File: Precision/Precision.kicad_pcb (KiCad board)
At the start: 2 copper layers, 76.2 x 76.2 mm, 159 parts, among them J1 M04PTH, J2 M04PTH, J3 M06SIP, J4 M04PTH, J405 Conn_01x08, J406 Conn_01x08, J5 M06SIP, J6 M02PTH, U401 ATMEGA328P-AU, U501 FT232RL, U602 ZF7, Y401 16MHz

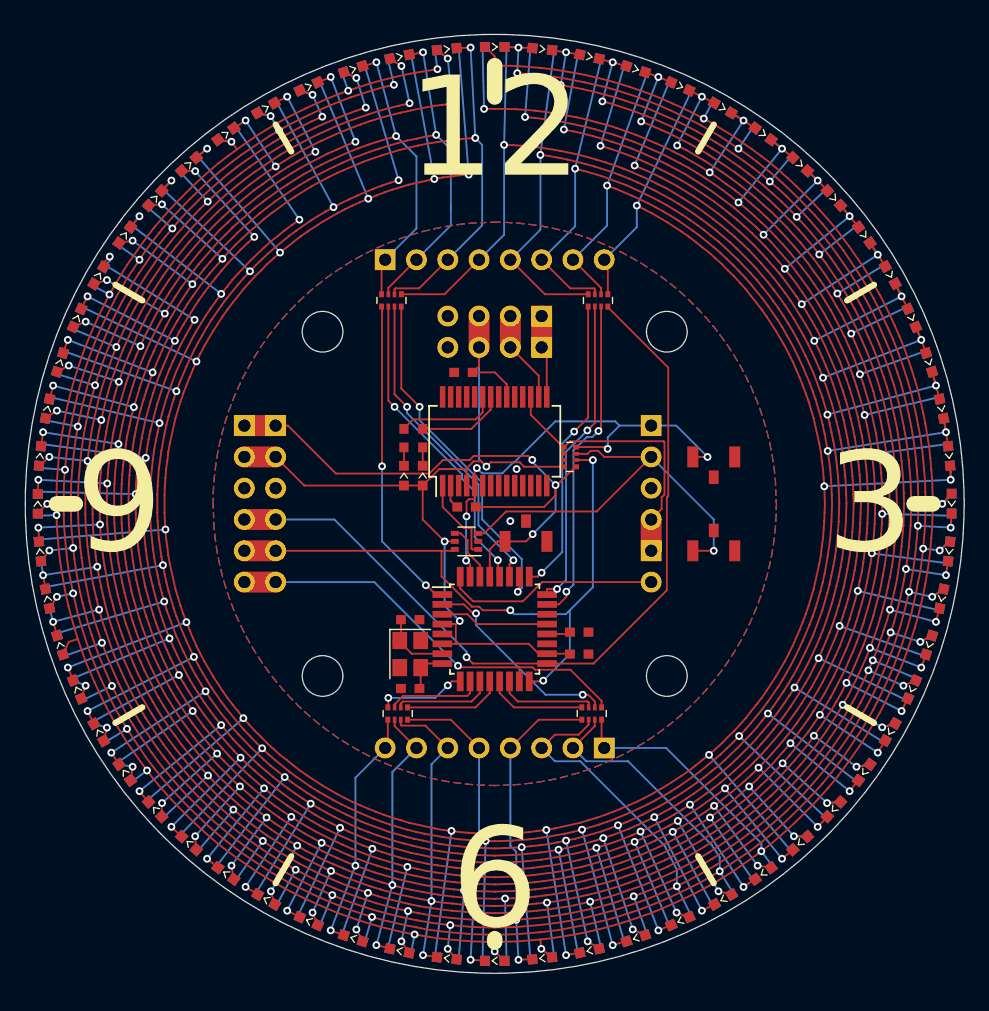
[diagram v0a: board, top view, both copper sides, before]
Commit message: j
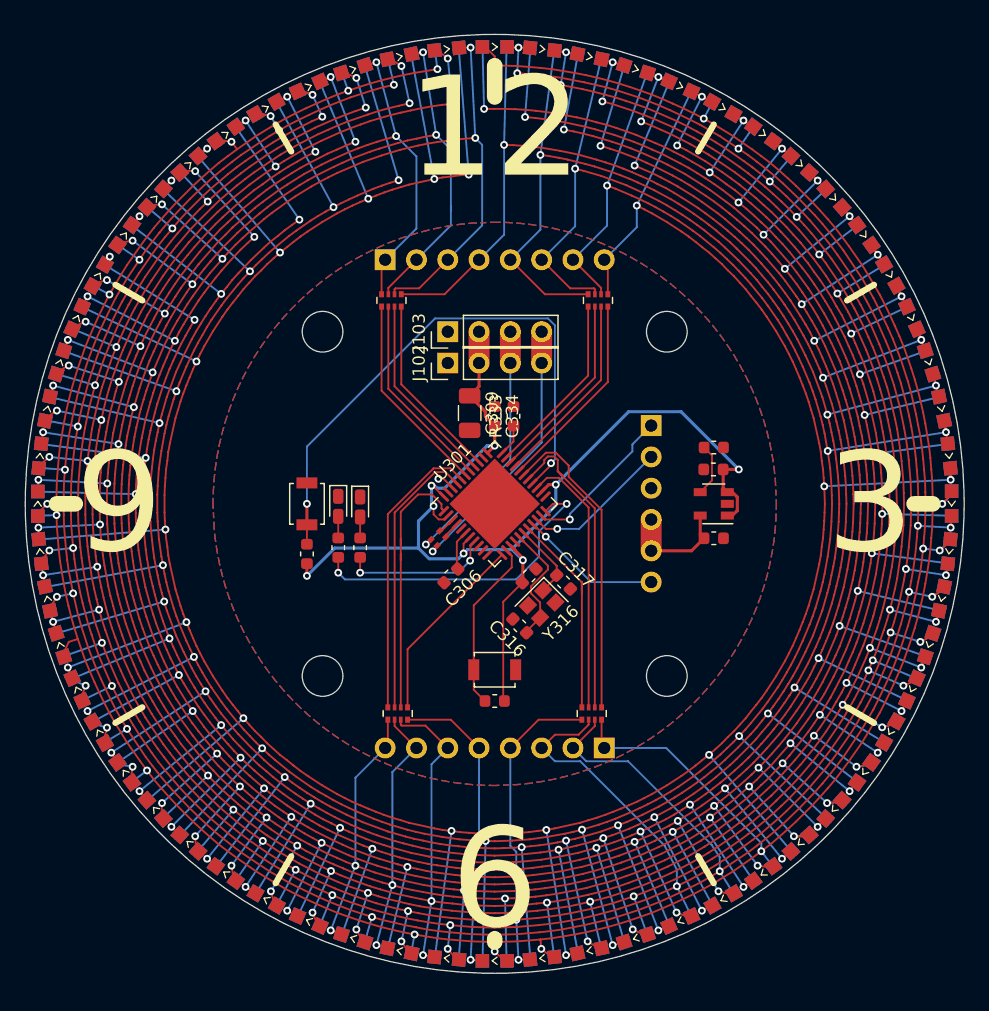
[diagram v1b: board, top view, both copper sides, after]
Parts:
- removed C10, C418: 4.7uF, KwanSystems:SMD_0603
- removed C407, C408: 18pF, KwanSystems:SMD_0603
- removed C420, C502: 100nF, KwanSystems:SMD_0603
- removed D501: BLUE, KwanSystems:D_0603
- removed D502: RED, KwanSystems:D_0603
- removed J1, J2: M04PTH, Connector_PinHeader_2.54mm:PinHeader_1x04_P2.54mm_Vertical
- removed J3, J5: M06SIP, Connector_PinHeader_2.54mm:PinHeader_1x06_P2.54mm_Vertical
- removed J6: M02PTH, Connector_PinHeader_2.54mm:PinHeader_1x02_P2.54mm_Vertical
- removed R501, R502: 680, KwanSystems:SMD_0603
- removed R606: 10k, KwanSystems:R_Array_Convex_4x0402
- removed REF**: KiCAD Logo, KwanSystems:Symbol_KiCAD-Logo_CopperAndSilkScreenTop_small
- removed REF**: OSHW-Symbol_6.7x6mm_SilkScreen, Symbol:OSHW-Symbol_6.7x6mm_SilkScreen
- removed REF**: StKwans, KwanSystems:ADivisionOf
- removed REF**: StKwans, KwanSystems:StKwans
- removed REF**: PrecisionKwan, KwanSystems:PrecisionKwan
- removed S429, S430, S431: B3U-1100P, KwanSystems:SW_SPST_B3U-1100P
- removed U501: FT232RL, Package_SO:SSOP-28_5.3x10.2mm_P0.65mm
- removed U602: ZF7, Package_TO_SOT_SMD:SOT-363_SC-70-6
- removed Y401: 16MHz, Crystal:Crystal_SMD_Abracon_ABM8G-4Pin_3.2x2.5mm
- added C306: 1uF, Capacitor_SMD:C_0603_1608Metric, F.Cu at (47.2, 56.6)
- added C309: 10uF, Capacitor_SMD:C_1206_3216Metric, F.Cu at (48.8, 43.4)
- added C314: 100nF, Capacitor_SMD:C_0603_1608Metric, F.Cu at (53.6, 56.6)
- added C316: 22pF, Capacitor_SMD:C_0603_1608Metric, F.Cu at (52.8, 60.7)
- added C317: 22pF, Capacitor_SMD:C_0603_1608Metric, F.Cu at (56.4, 57.1)
- added C334: 100nF, Capacitor_SMD:C_0603_1608Metric, F.Cu at (50.8, 43.7)
- added C401: 1uF, Capacitor_SMD:C_0603_1608Metric, F.Cu at (68.6, 48.0)
- added C404: 100nF, Capacitor_SMD:C_0603_1608Metric, F.Cu at (68.6, 46.2)
- added C405: 2.2uF, Capacitor_SMD:C_0603_1608Metric, F.Cu at (68.6, 53.6)
- added D308: RED, LED_SMD:LED_0603_1608Metric_Castellated, F.Cu at (39.9, 51.1)
- added D322: green, LED_SMD:LED_0603_1608Metric_Castellated, F.Cu at (38.1, 51.0)
- added G101: KwanSystems, KwanSystems:PrecisionKwan, B.Cu at (50.8, 50.8)
- added G102: DesignedWithKicad, KwanSystems:Symbol_KiCAD-Logo_CopperAndSilkScreenTop_small, B.Cu at (30.0, 60.2)
- added J102: M04PTH, Connector_PinHeader_2.54mm:PinHeader_1x04_P2.54mm_Vertical, F.Cu at (47.0, 39.4)
- added J103: M04PTH, Connector_PinHeader_2.54mm:PinHeader_1x04_P2.54mm_Vertical, F.Cu at (47.0, 36.8)
- added R101: 10k, Resistor_SMD:R_0603_1608Metric, F.Cu at (35.6, 54.9)
- added R303: 22, KwanSystems:R_Array_Convex_2x0402, F.Cu at (46.2, 53.6)
- added R308: 1k, Resistor_SMD:R_0603_1608Metric, F.Cu at (39.9, 54.4)
- added R313: 10k, Resistor_SMD:R_0603_1608Metric, F.Cu at (50.8, 66.8)
- added R322: 1k, Resistor_SMD:R_0603_1608Metric, F.Cu at (38.1, 54.4)
- added R333: 10k, Resistor_SMD:R_0603_1608Metric, F.Cu at (52.3, 43.7)
- added S102: B3U-1000P, KwanSystems:SW_SPST_B3U-1000P, F.Cu at (35.6, 50.8)
- added S313: RESET, KwanSystems:SW_SPST_B3U-1000P, F.Cu at (50.8, 64.3)
- added U301: ATmega32U4-MU, Package_DFN_QFN:QFN-44-1EP_7x7mm_P0.5mm_EP5.2x5.2mm, F.Cu at (50.8, 50.8)
- added Y316: 16MHz, Crystal:Crystal_SMD_2520-4Pin_2.5x2.0mm, F.Cu at (54.6, 58.9)
- D000, D001, D002, D003, D004, D005, D006, D007, D008, D009, D010, D011, D012, D013, D014, D015, D016, D017, D018, D019, D020, D021, D022, D023, D024, D025, D026, D027, D028, D029, D030, D031, D032, D033, D034, D035, D036, D037, D038, D039, D040, D041, D042, D043, D044, D045, D046, D047, D048, D049, D050, D051, D052, D053, D054, D055, D056, D057, D058, D059, D100, D101, D102, D103, D104, D105, D106, D107, D108, D109, D110, D111, D112, D113, D114, D115, D116, D117, D118, D119, D120, D121, D122, D123, D124, D125, D126, D127, D128, D129, D130, D131, D132, D133, D134, D135, D136, D137, D138, D139, D140, D141, D142, D143, D144, D145, D146, D147, D148, D149, D150, D151, D152, D153, D154, D155, D156, D157, D158, D159: footprint KwanSystems:D_0603 -> KwanSystems:D_0603_SIDE
- J101: renamed from J4; value M04PTH -> M06PTH; footprint Connector_PinHeader_2.54mm:PinHeader_1x04_P2.54mm_Vertical -> Connector_PinHeader_2.54mm:PinHeader_1x06_P2.54mm_Vertical
- U401: value ATMEGA328P-AU -> MIC5319 3.3V; footprint Package_QFP:TQFP-32_7x7mm_P0.8mm -> Package_TO_SOT_SMD:SOT-23-5
- moved U401 20.5 mm to (68.6, 50.8), turned to 180 degrees
- renumbered J405 to J104, J406 to J105, JP1 to JP101, JP2 to JP102, JP3 to JP103, JP4 to JP104, R4 to R102, R3 to R103, R2 to R104, R1 to R105
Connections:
- J101 pad 1: /AT_TX -> /GPS_RX
- U401 pad 1: /P09 -> VBUS
- U401 pad 2: /P02 -> GND
- U401 pad 3: GND -> VBUS
- U401 pad 4: +5V -> /3.3V Regulator/BYP
- U401 pad 5: GND -> +3V3
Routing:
- net VBUS: track 0.00 -> 98.9 mm, vias 0 -> 8
- net +5V: track 77.4 -> 0.00 mm, vias 3 -> 0
- net /D12: track 53.1 -> 0.00 mm, vias 3 -> 0
- net /P16: track 67.0 -> 16.3 mm, vias 1 -> 0
- net /RESET: track 49.5 -> 0.00 mm, vias 3 -> 0
- net /SET: track 0.00 -> 46.2 mm, vias 0 -> 2
- net /AT_TX: track 37.5 -> 0.00 mm, vias 5 -> 0
- net /Arduino 32U4/TXLED: track 0.00 -> 25.7 mm, vias 0 -> 2
- net /GPS_TX: track 34.4 -> 12.0 mm
- net /D+: track 0.00 -> 22.1 mm, vias 0 -> 1
- net /D-: track 0.00 -> 20.7 mm, vias 0 -> 1
- net /P08: track 7.18 -> 23.5 mm, vias 2 -> 0
- net /P07: track 7.70 -> 22.6 mm
- net +3V3: track 23.5 -> 9.23 mm
- net /Arduino 32U4/RESET: track 0.00 -> 14.1 mm
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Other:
- board text added: "25 Dec 2020"
- board text removed: "25 Dec 2019"
